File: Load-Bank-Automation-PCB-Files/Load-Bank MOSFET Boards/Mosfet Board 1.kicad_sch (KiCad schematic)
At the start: 27 parts, among them J1 Conn_02x03_Counter_Clockwise, Q22 GSGN0648, Q3 GSGN0648, U10 MCP6006-OTVAO, U7 ACS711KEXLT-31AB-T, U8 IRS10752LTRPBF

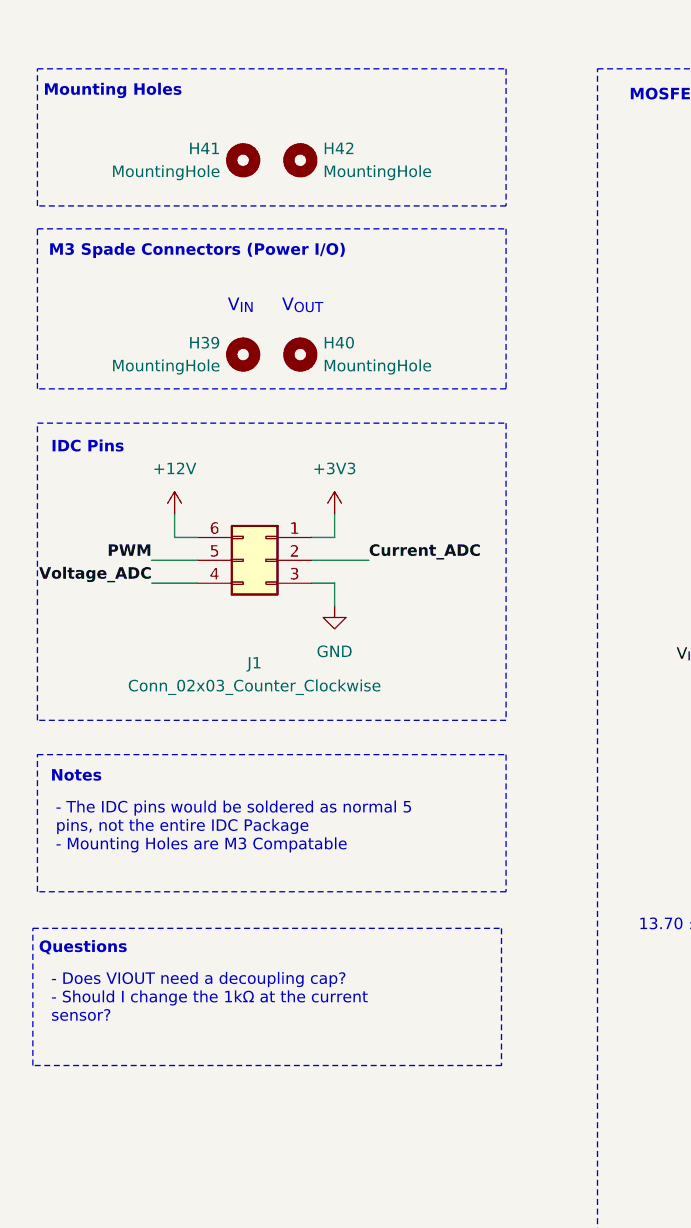
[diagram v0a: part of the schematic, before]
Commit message: A
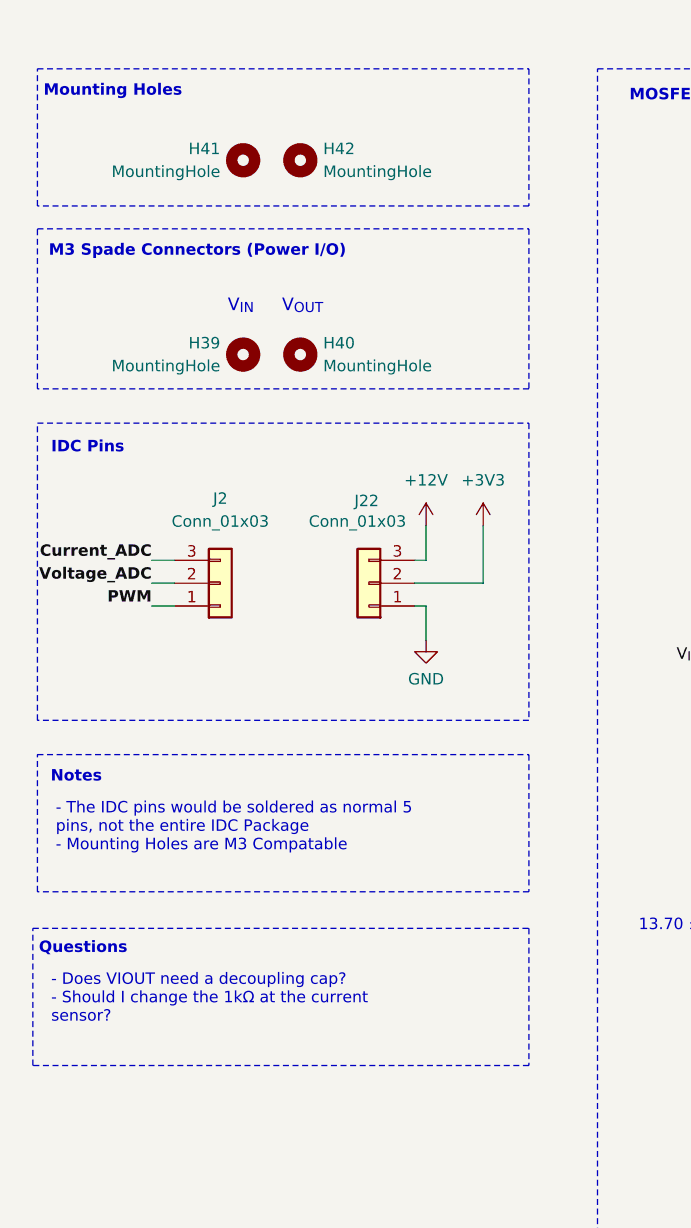
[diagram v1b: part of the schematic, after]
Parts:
- removed J1: Conn_02x03_Counter_Clockwise, Connector_IDC:IDC-Header_2x03_P2.54mm_Vertical, symbol Connector_Generic:Conn_02x03_Counter_Clockwise
- added J2, J22: Conn_01x03, Connector_PinHeader_1.00mm:IDC_PinHeader_1x03_P1.00mm_Vertical, symbol Connector_Generic:Conn_01x03
- H41, H42: footprint TerminalBlock_MetzConnect:TerminalBlock_MetzConnect_360271_1x01_Horizontal_ScrewM3.0_Boxed -> MountingHole:MountingHole_3.2mm_M3
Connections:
- net +12V: now also J22.3 (Pin_3)
- net +3V3: now also J22.2 (Pin_2)
- net Current_ADC: now also J2.3 (Pin_3)
- net GND: now also J22.1 (Pin_1)
- net PWM: now also J2.1 (Pin_1)
- net Voltage_ADC: now also J2.2 (Pin_2)
